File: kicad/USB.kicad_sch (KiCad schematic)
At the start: 7 parts, among them CN1 SHOU-HAN-TYPE-C16PIN_C393939

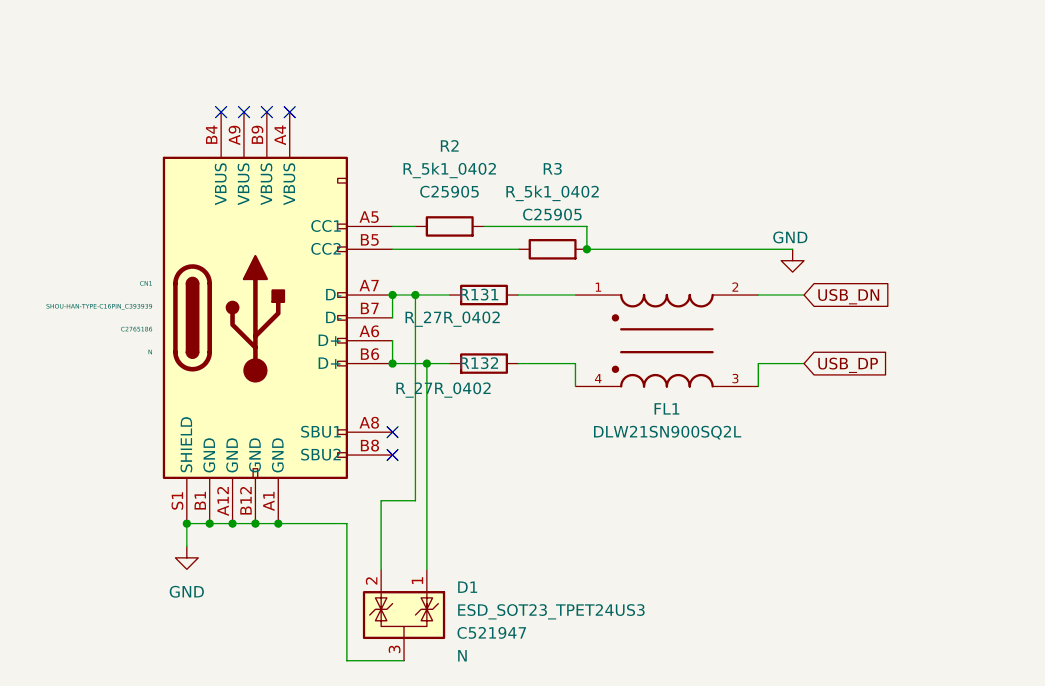
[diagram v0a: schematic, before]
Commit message: sch done-ish
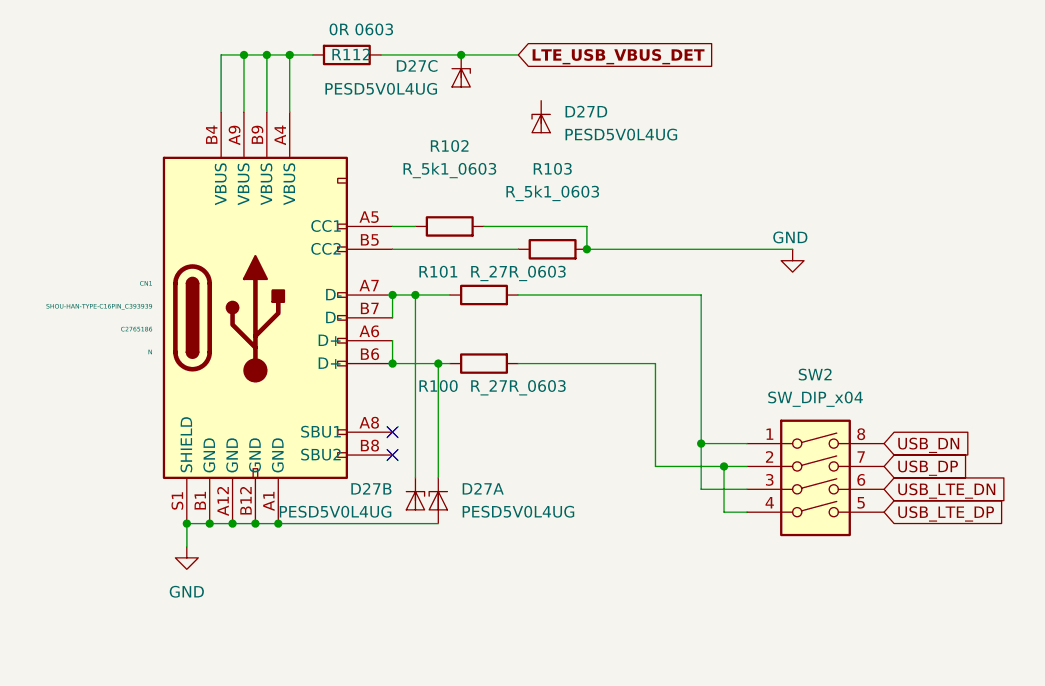
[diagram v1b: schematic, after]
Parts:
- removed D1: ESD_SOT23_TPET24US3, Package_TO_SOT_SMD:SOT-23, symbol Skrubis:ESD_SOT23_TPET24US3
- removed FL1: DLW21SN900SQ2L, sensehalo:FIL_DLW21SN900SQ2L, symbol sensehalo:DLW21SN900SQ2L
- removed R131, R132: R_27R_0402, Resistor_SMD:R_0402_1005Metric, symbol Skrubis:R_1M_0603
- removed R2, R3: R_5k1_0402, Resistor_SMD:R_0402_1005Metric, symbol Skrubis:R_5k1_0603
- added D27: PESD5V0L4UG, Package_TO_SOT_SMD:SOT-353_SC-70-5, symbol Power_Protection:PESD5V0L4UG
- added R100, R101: R_27R_0603, Resistor_SMD:R_0603_1608Metric, symbol Skrubis:R_27R_0603
- added R102, R103: R_5k1_0603, Resistor_SMD:R_0603_1608Metric, symbol Skrubis:R_5k1_0603
- added R112: 0R 0603, Resistor_SMD:R_0603_1608Metric, symbol Device:R
- added SW2: SW_DIP_x04, Button_Switch_THT:SW_DIP_SPSTx04_Slide_9.78x12.34mm_W7.62mm_P2.54mm, symbol Switch:SW_DIP_x04
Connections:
- net GND: now also D27.2 (A), R102.2, R103.2
- net USB_DN: now also SW2.8
- net USB_DP: now also SW2.7
- net at CN1.A7 (D-), CN1.B7 (D-): now also D27.3 (K2), R101.1
- net at CN1.A4 (VBUS): now also CN1.A9 (VBUS), CN1.B4 (VBUS), CN1.B9 (VBUS), R112.2
- net at CN1.A5 (CC1): now also R102.1
- net at CN1.A6 (D+), CN1.B6 (D+): now also D27.1 (K1), R100.1
- net at CN1.B5 (CC2): now also R103.1
- new net: R100.2, SW2.2, SW2.4
- new net: R101.2, SW2.1, SW2.3
- new net LTE_USB_VBUS_DET: D27.4 (K3), R112.1
- new net USB_LTE_DN: SW2.6
- new net USB_LTE_DP: SW2.5
- no-connect marks 6 -> 2
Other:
- company: (none) -> ©CC-BY-NC
- title: (none) -> VehicleMan

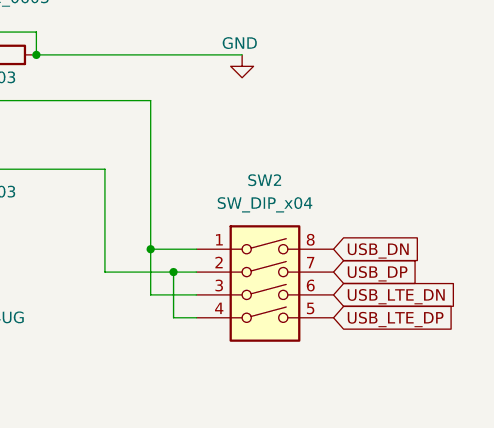
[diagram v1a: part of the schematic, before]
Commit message: WIP
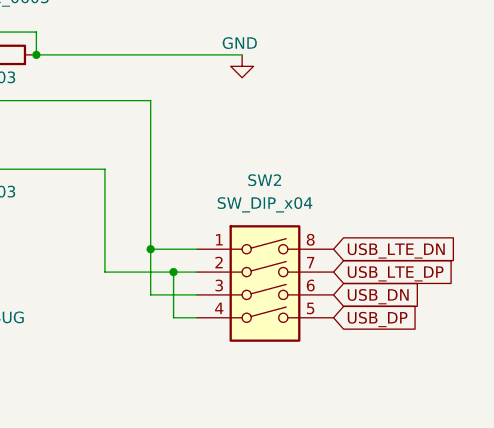
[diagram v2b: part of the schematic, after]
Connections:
- net USB_DN: now also SW2.6; no longer SW2.8
- net USB_DP: now also SW2.5; no longer SW2.7
- net USB_LTE_DN: now also SW2.8; no longer SW2.6
- net USB_LTE_DP: now also SW2.7; no longer SW2.5
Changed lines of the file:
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@@
 		)
 	)
-	(global_label "USB_LTE_DN"
+	(global_label "USB_DP"
+		(shape input)
+		(at 121.92 90.17 0)
+		(fields_autoplaced yes)
+		(effects
+			(font
+				(size 1.27 1.27)
+			)
+			(justify left)
+		)
+		(property "Intersheetrefs" "${INTERSHEET_REFS}"
+			(at 131.6507 90.0906 0)
+			(effects
+				(font
+					(size 1.27 1.27)
+				)
+				(justify left)
+				(hide yes)
+			)
+		)
+	)
+	(global_label "USB_DN"
 		(shape input)
 		(at 121.92 87.63 0)
@@
 		)
 		(property "Intersheetrefs" "${INTERSHEET_REFS}"
-			(at 136.3956 87.63 0)
+			(at 131.7112 87.5506 0)
+			(effects
+				(font
+					(size 1.27 1.27)
+				)
+				(justify left)
+				(hide yes)
+			)
+		)
+	)
+	(global_label "USB_LTE_DN"
+		(shape input)
+		(at 121.92 82.55 0)
+		(fields_autoplaced yes)
+		(effects
+			(font
+				(size 1.27 1.27)
+			)
+			(justify left)
+		)
+		(property "Intersheetrefs" "${INTERSHEET_REFS}"
+			(at 136.3956 82.55 0)
 			(effects
 				(font
@@
 	(global_label "USB_LTE_DP"
 		(shape input)
-		(at 121.92 90.17 0)
-		(fields_autoplaced yes)
-		(effects
-			(font
-				(size 1.27 1.27)
-			)
-			(justify left)
-		)
-		(property "Intersheetrefs" "${INTERSHEET_REFS}"
-			(at 136.3351 90.17 0)
-			(effects
-				(font
-					(size 1.27 1.27)
-				)
-				(justify left)
-				(hide yes)
-			)
-		)
-	)
-	(global_label "USB_DN"
-		(shape input)
-		(at 121.92 82.55 0)
-		(fields_autoplaced yes)
-		(effects
-			(font
-				(size 1.27 1.27)
-			)
-			(justify left)
-		)
-		(property "Intersheetrefs" "${INTERSHEET_REFS}"
-			(at 131.7112 82.4706 0)
-			(effects
-				(font
-					(size 1.27 1.27)
-				)
-				(justify left)
-				(hide yes)
-			)
-		)
-	)
-	(global_label "USB_DP"
-		(shape input)
 		(at 121.92 85.09 0)
 		(fields_autoplaced yes)
@@
 		)
 		(property "Intersheetrefs" "${INTERSHEET_REFS}"
-			(at 131.6507 85.0106 0)
+			(at 136.3351 85.09 0)
 			(effects
 				(font
